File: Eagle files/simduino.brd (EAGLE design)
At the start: 69.5 x 54.6 mm, 15 parts, among them IC1 ATMEGA168-20P, Q1 16MHz

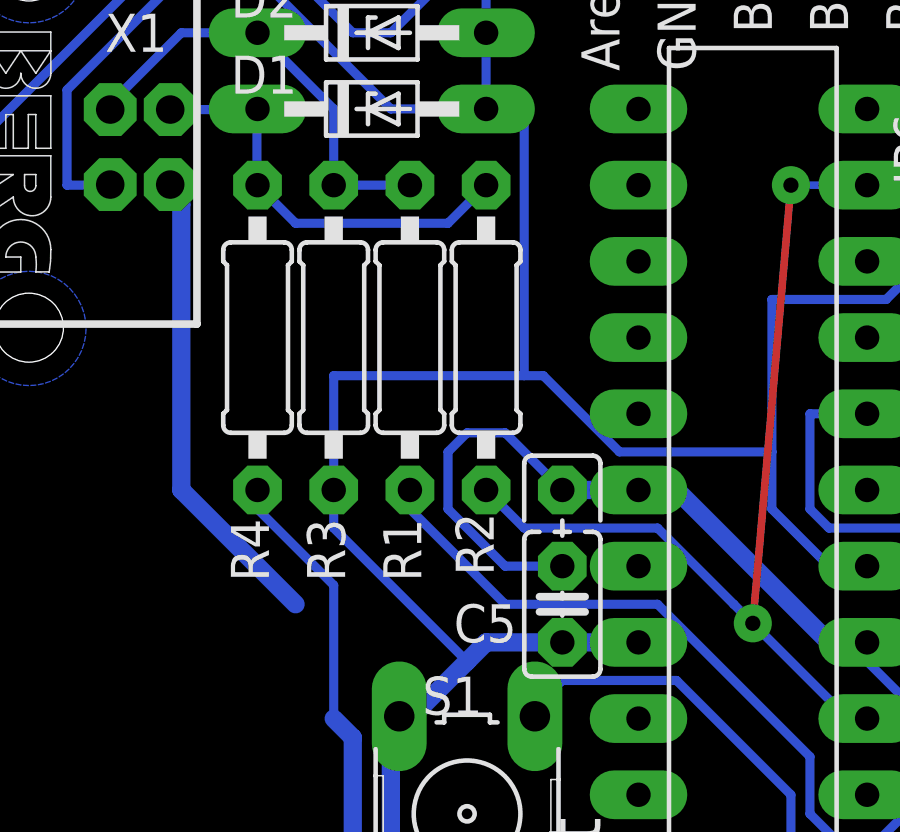
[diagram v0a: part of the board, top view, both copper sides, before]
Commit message: Streamlining
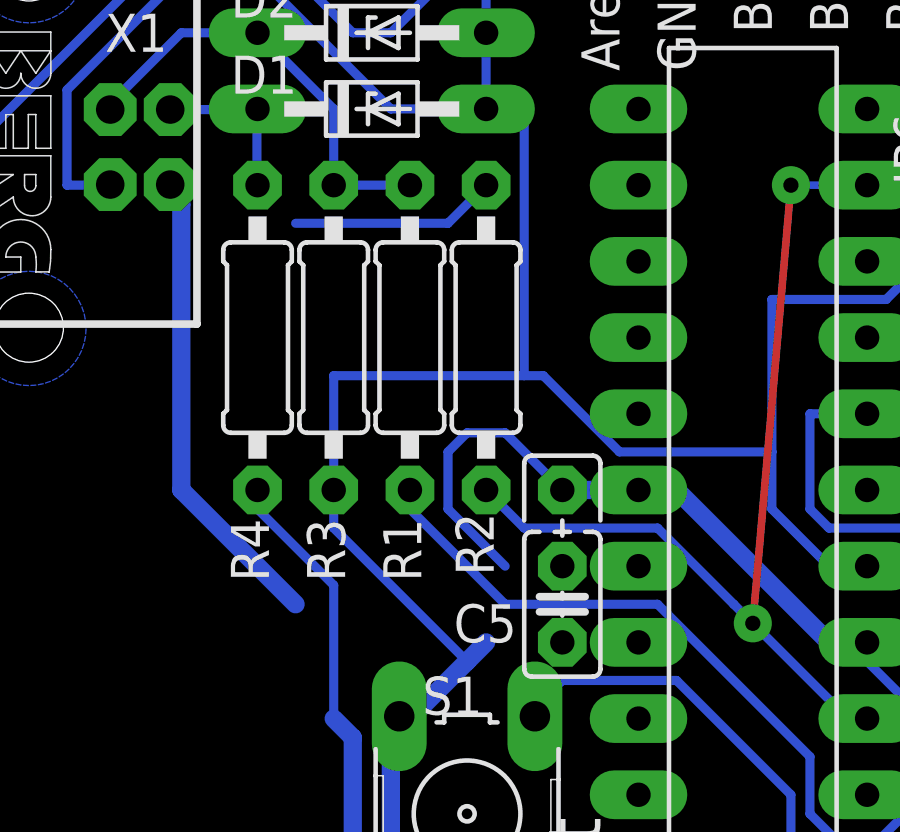
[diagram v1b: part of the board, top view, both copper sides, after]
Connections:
- net +5USB: now also C5.1; no longer C5.2
- net GND: now also C5.2; no longer C5.1
- net N$2: now also S1.3
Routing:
- net GND: track 125.3 -> 120.2 mm
- net +5USB: track 230.7 -> 228.2 mm
- net D-: track 14.1 -> 12.3 mm
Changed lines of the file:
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@@
 <wire x1="8.89" y1="31.75" x2="8.89" y2="41.275" width="0.6096" layer="16"/>
 <wire x1="8.89" y1="41.275" x2="8.52" y2="41.93" width="0.6096" layer="16"/>
-<contactref element="C5" pad="2"/>
 <contactref element="IC1" pad="20"/>
 <contactref element="IC1" pad="7"/>
 <contactref element="C2" pad="+"/>
-<contactref element="R4" pad="1"/>
 <wire x1="25.4" y1="31.75" x2="24.13" y2="31.75" width="0.6096" layer="16"/>
 <wire x1="30.48" y1="26.67" x2="25.4" y2="31.75" width="0.6096" layer="16"/>
@@
 <wire x1="13.97" y1="24.13" x2="13.97" y2="28.575" width="0.3048" layer="16"/>
 <wire x1="13.97" y1="28.575" x2="11.43" y2="31.115" width="0.3048" layer="16"/>
-<wire x1="11.43" y1="31.115" x2="11.43" y2="31.75" width="0.3048" layer="16"/>
-<wire x1="19.685" y1="29.21" x2="21.59" y2="29.21" width="0.3048" layer="16"/>
 <wire x1="17.78" y1="31.115" x2="19.685" y2="29.21" width="0.3048" layer="16"/>
 <wire x1="17.78" y1="33.02" x2="17.78" y2="31.115" width="0.3048" layer="16"/>
@@
 <wire x1="21.59" y1="31.75" x2="19.685" y2="33.655" width="0.3048" layer="16"/>
 <wire x1="24.13" y1="31.75" x2="21.59" y2="31.75" width="0.6096" layer="16"/>
-<wire x1="13.97" y1="28.575" x2="12.7" y2="27.94" width="0" layer="19" extent="16-16"/>
-<wire x1="17.78" y1="31.115" x2="13.97" y2="28.575" width="0" layer="19" extent="16-16"/>
+<contactref element="C5" pad="1"/>
+<contactref element="R4" pad="1"/>
+<wire x1="19.685" y1="29.21" x2="21.59" y2="26.67" width="0" layer="19" extent="16-16"/>
+<wire x1="13.97" y1="28.575" x2="17.78" y2="31.115" width="0" layer="19" extent="16-16"/>
+<wire x1="11.43" y1="31.75" x2="11.43" y2="31.115" width="0" layer="19" extent="16-16"/>
+<wire x1="12.7" y1="27.94" x2="13.97" y2="28.575" width="0" layer="19" extent="16-16"/>
 </signal>
 <signal name="N$2">
@@
 <wire x1="21.59" y1="25.4" x2="20.955" y2="24.765" width="0.3048" layer="16"/>
 <wire x1="20.955" y1="24.765" x2="20.6756" y2="24.2062" width="0.3048" layer="16"/>
+<contactref element="S1" pad="3"/>
+<wire x1="20.6756" y1="17.7038" x2="20.6756" y2="24.2062" width="0" layer="19" extent="1-1"/>
 </signal>
 <signal name="N$5">
@@
 <contactref element="R2" pad="1"/>
 <contactref element="D1" pad="C"/>
-<contactref element="R4" pad="2"/>
-<wire x1="11.43" y1="41.91" x2="12.7" y2="40.64" width="0.3048" layer="16"/>
 <wire x1="12.7" y1="40.64" x2="17.78" y2="40.64" width="0.3048" layer="16"/>
 <wire x1="17.78" y1="40.64" x2="19.05" y2="41.91" width="0.3048" layer="16"/>
@@
 <wire x1="11.41" y1="44.43" x2="11.43" y2="44.45" width="0.3048" layer="16"/>
 <wire x1="11.41" y1="41.93" x2="11.41" y2="44.43" width="0.3048" layer="16"/>
-<wire x1="11.43" y1="41.91" x2="11.41" y2="41.93" width="0.3048" layer="16"/>
+<contactref element="R4" pad="2"/>
+<wire x1="11.43" y1="41.91" x2="12.7" y2="40.64" width="0" layer="19" extent="16-16"/>
+<wire x1="11.41" y1="41.93" x2="11.43" y2="41.91" width="0" layer="19" extent="16-16"/>
 </signal>
 <signal name="D+">
@@
 <contactref element="S1" pad="2"/>
 <contactref element="IC1" pad="22"/>
-<contactref element="C5" pad="1"/>
 <contactref element="S1" pad="1"/>
 <contactref element="C2" pad="-"/>
@@
 <contactref element="X1" pad="4"/>
 <contactref element="R3" pad="1"/>
-<wire x1="21.59" y1="26.67" x2="24.13" y2="26.67" width="0.6096" layer="16"/>
-<wire x1="19.05" y1="26.67" x2="21.59" y2="26.67" width="0.6096" layer="16"/>
 <wire x1="16.4338" y1="24.2062" x2="16.1544" y2="24.2062" width="0.6096" layer="16"/>
 <wire x1="16.51" y1="24.13" x2="16.4338" y2="24.2062" width="0.6096" layer="16"/>
@@
 <vertex x="-0.635" y="-0.635"/>
 </polygon>
+<contactref element="C5" pad="2"/>
+<wire x1="21.59" y1="29.21" x2="24.13" y2="26.67" width="0" layer="19" extent="1-1"/>
+<wire x1="19.05" y1="26.67" x2="21.59" y2="29.21" width="0" layer="19" extent="16-16"/>
 </signal>
 <signal name="N$188">

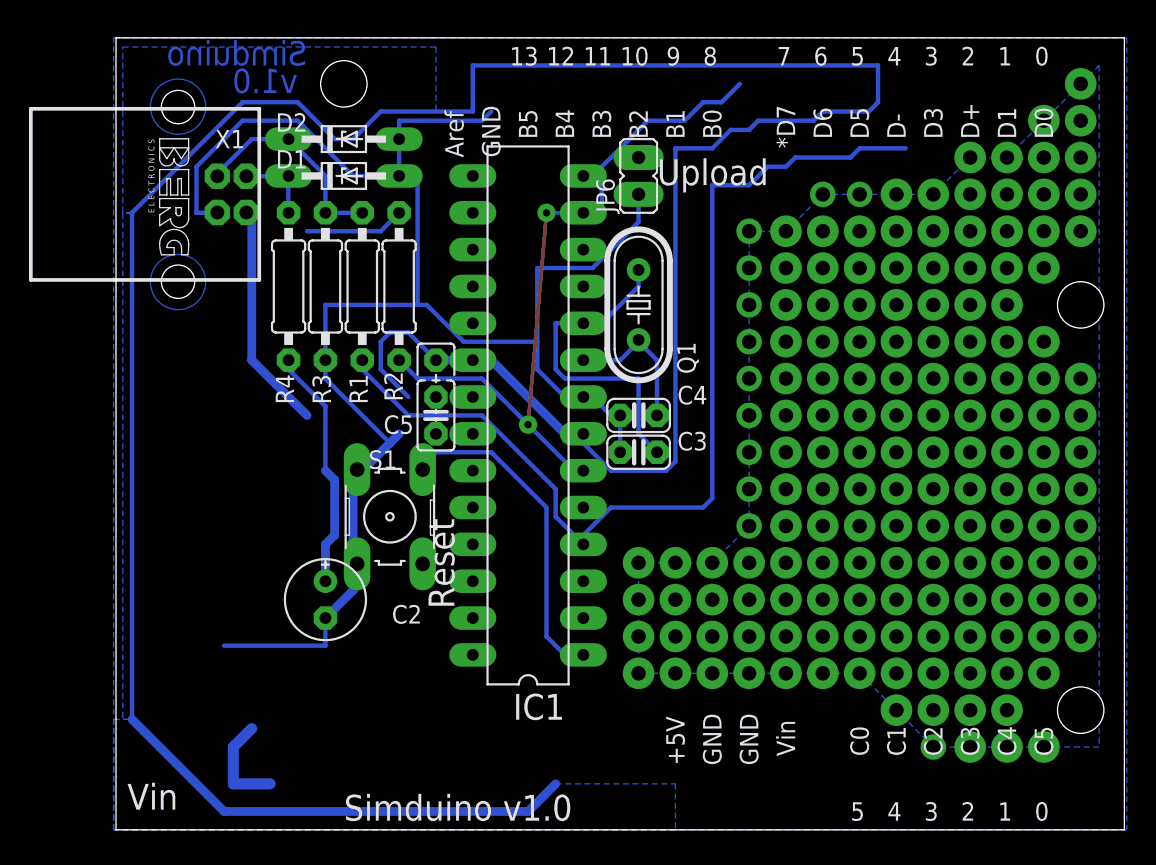
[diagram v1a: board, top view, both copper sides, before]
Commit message: Cleanup
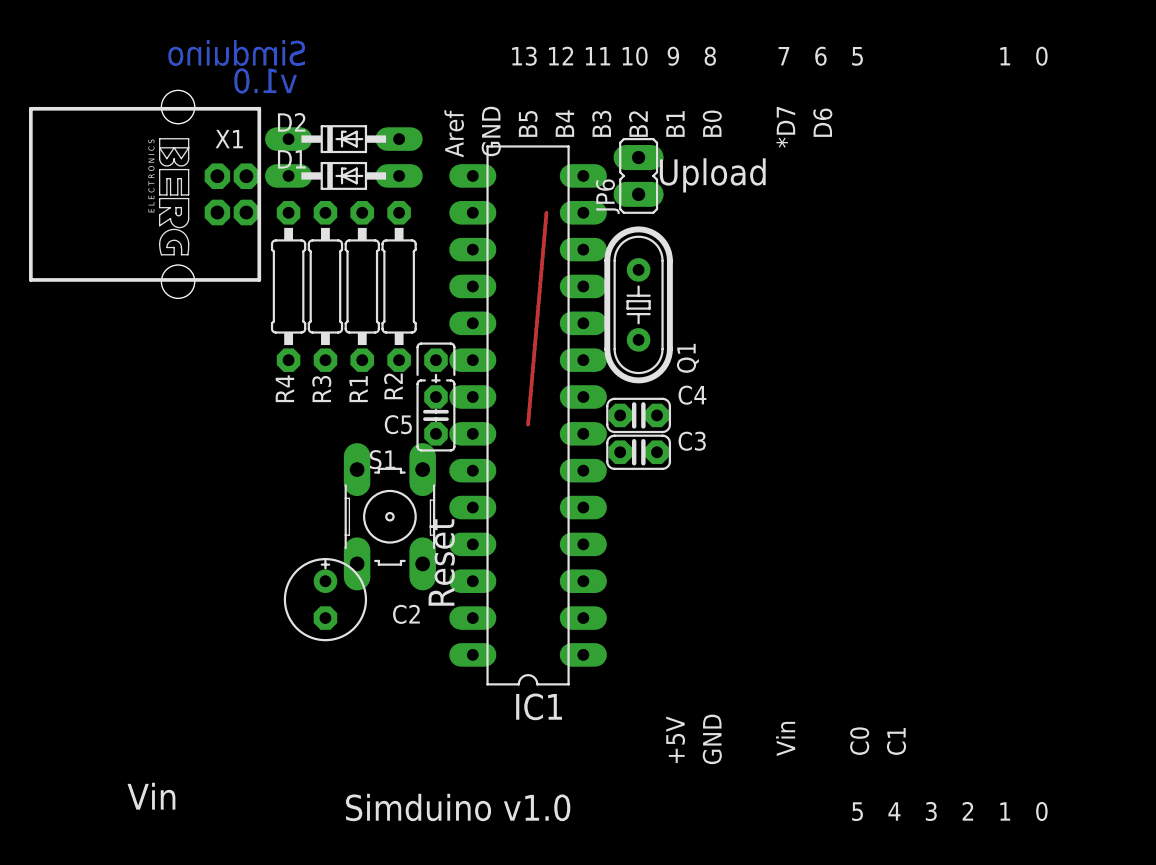
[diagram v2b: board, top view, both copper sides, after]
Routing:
- net +5USB: track 228.2 -> 0.00 mm
- net GND: track 120.2 -> 0.00 mm
- net N$3: track 68.5 -> 0.00 mm
- net N$1: track 50.3 -> 14.7 mm, vias 2 -> 0
- net N$9: track 22.8 -> 0.00 mm
- net N$2: track 22.7 -> 0.00 mm
- net D+: track 14.8 -> 0.00 mm
- net D-: track 12.3 -> 0.00 mm
- net N$10: track 10.1 -> 0.00 mm
- net N$15: track 6.88 -> 0.00 mm
- removed copper zone on layer 16, net +5V
- removed copper zone on layer 16, net GND
- removed copper zone on layer 16, net N$187
- removed copper zone on layer 16, net N$188
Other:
- board outline removed
- board text removed: "C2"
- board text removed: "C3"
- board text removed: "C4"
- board text removed: "C5"
- board text removed: "D+"
- board text removed: "D-"
- board text removed: "D0"
- board text removed: "D1"
- board text removed: "D3"
- board text removed: "D5"
